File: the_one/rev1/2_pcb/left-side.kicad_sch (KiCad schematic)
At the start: 39 parts, among them SW1 KeySwitch, SW10 KeySwitch, SW11 KeySwitch, SW12 KeySwitch, SW13 KeySwitch, SW14 KeySwitch, SW15 KeySwitch, SW16 KeySwitch, SW17 KeySwitch, SW18 KeySwitch, SW19 KeySwitch, SW2 KeySwitch, SW3 KeySwitch, SW4 KeySwitch, SW5 KeySwitch, SW6 KeySwitch, SW7 KeySwitch, SW8 KeySwitch, SW9 KeySwitch, U1 Pico

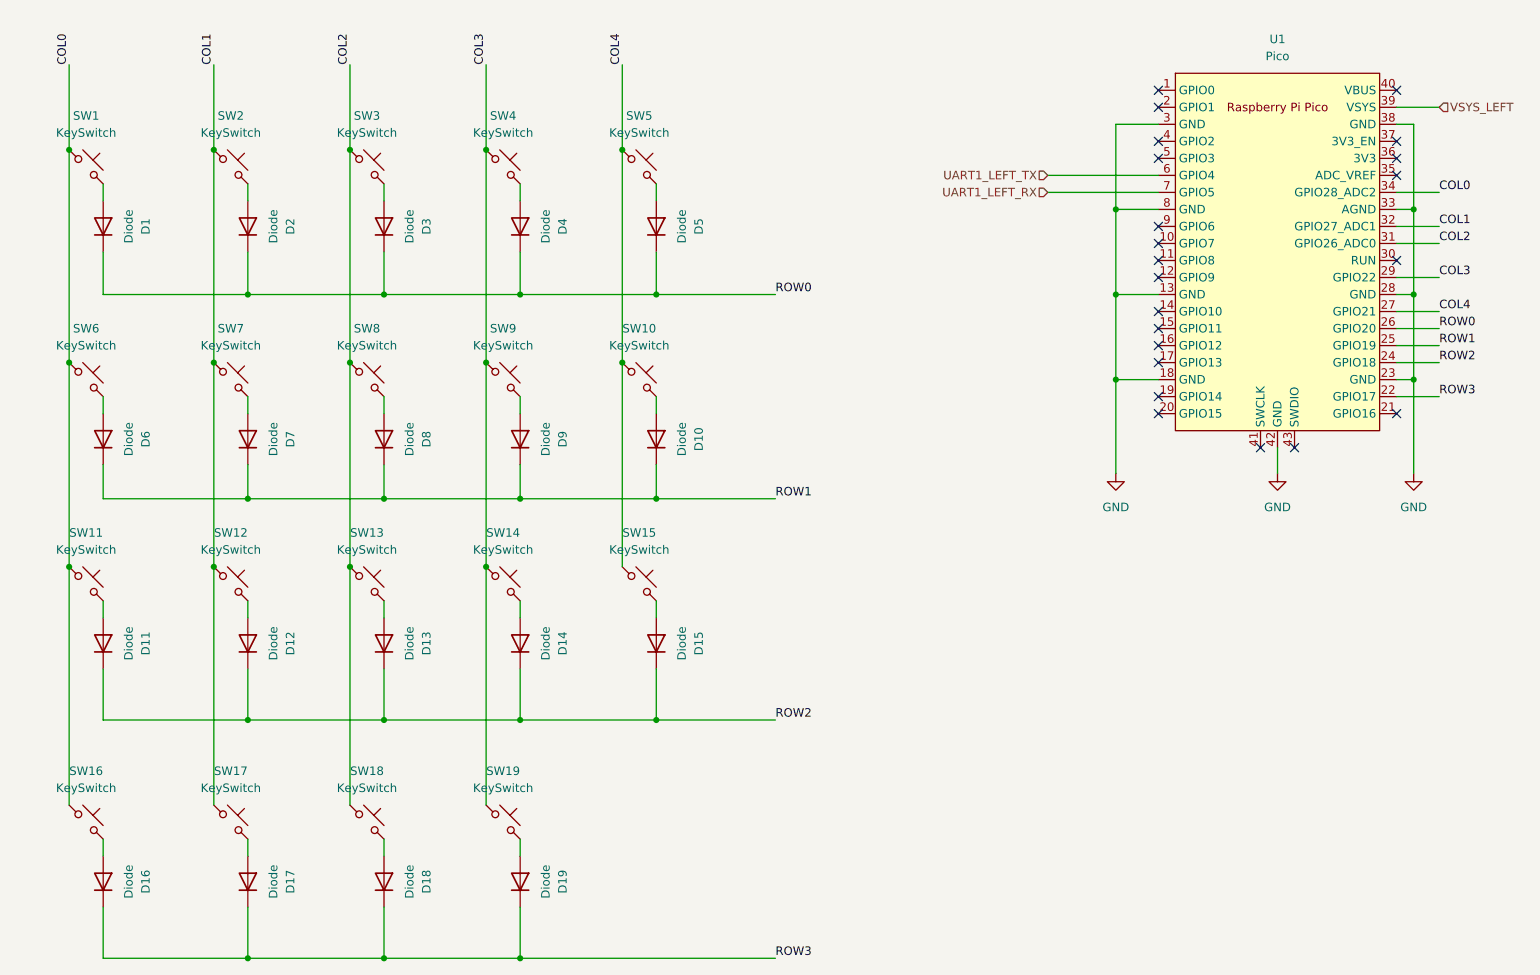
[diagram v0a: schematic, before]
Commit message: update KiCAD schematcis
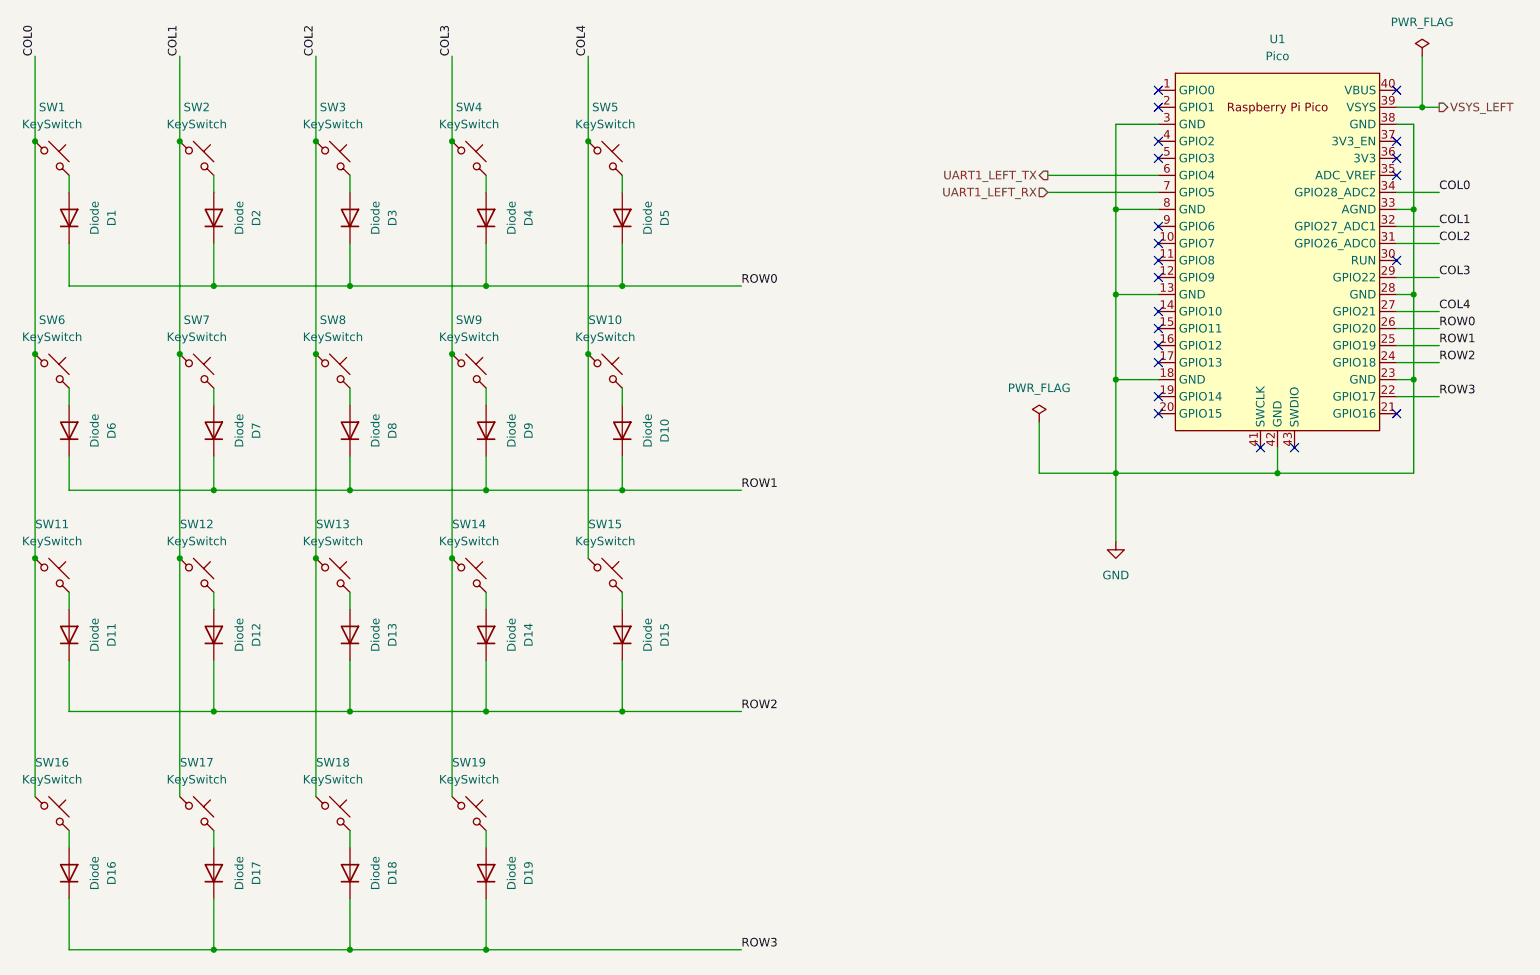
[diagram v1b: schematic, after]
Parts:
- U1: footprint RPi_Pico:RPi_Pico_SMD_TH -> MCU_RaspberryPi_and_Boards:RPi_Pico_SMD_TH
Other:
- moved on the sheet: D1, D10, D11, D12, D13, D14, D15, D16, D17, D18, D19, D2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
